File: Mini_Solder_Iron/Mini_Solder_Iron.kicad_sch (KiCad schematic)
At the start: 89 parts, among them CN1 YXT-BB10-24S-02, J1 USB_C_Receptacle_USB2.0, J2 Negative, J3 Positive, J4 Conn_01x04, J5 Conn_01x04, J6 Conn_01x04, J7 Com, J8 Conn_01x04, Q1 AO4407A, Q2 MMBT3904, SW1 SW_Push, SW2 SW_Push, U1 STM32F103C8T6, U2 LIS2DS12, U3 SGM8557-1AXN5G/TR, U4 TMP36GRTZ, U5 CH340E, U6 MP9942, U7 CH224K, U8 LP5907MFX-3.3, U9 LP5907MFX-1.8, Y1 Crystal_GND3_Small

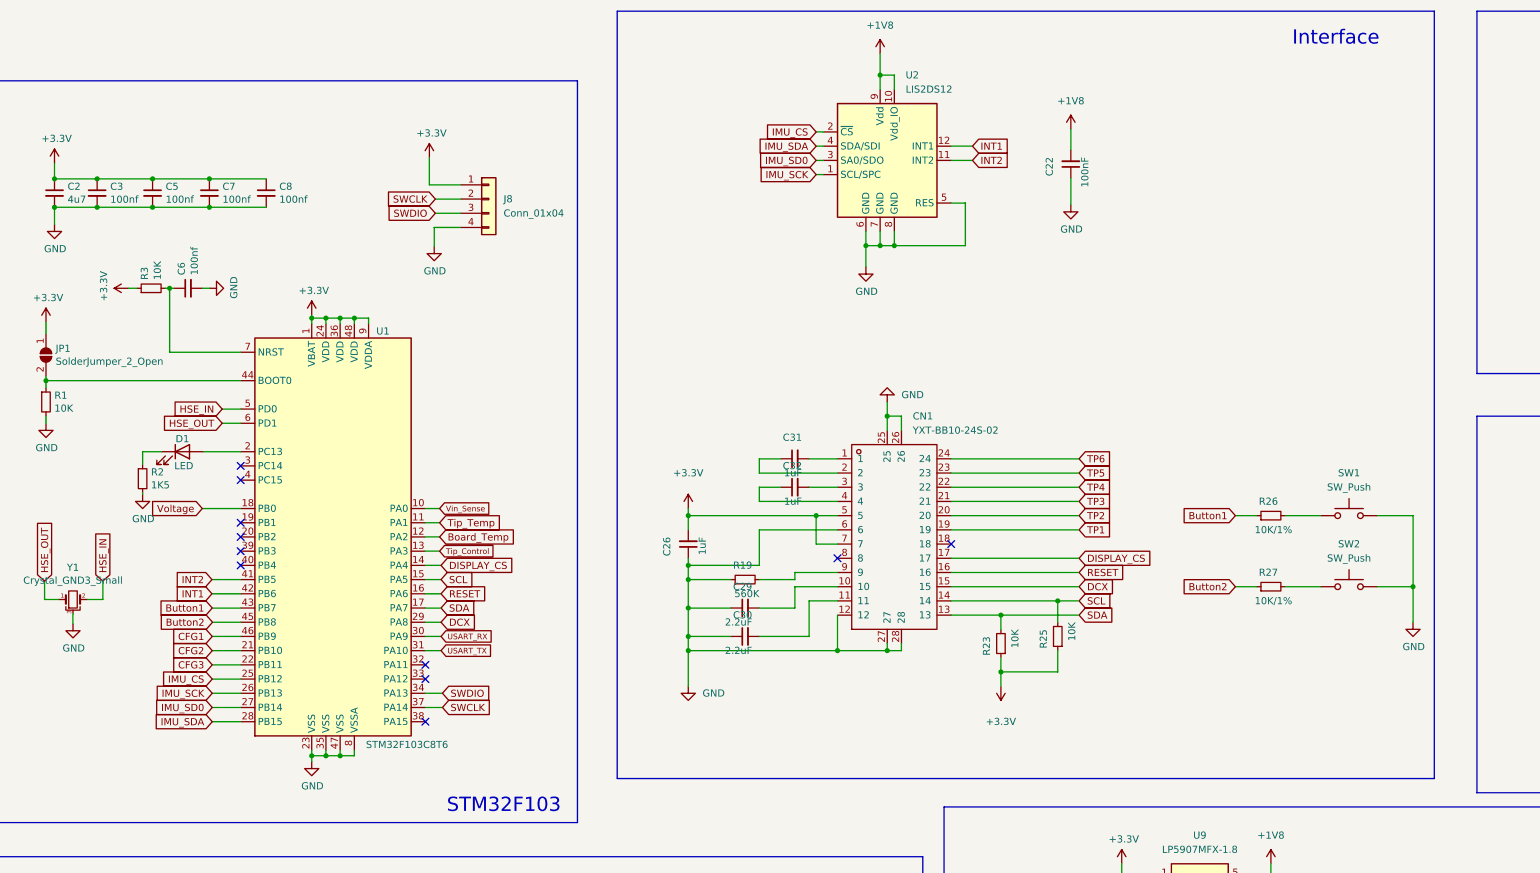
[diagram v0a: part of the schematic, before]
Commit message: PCB layout update
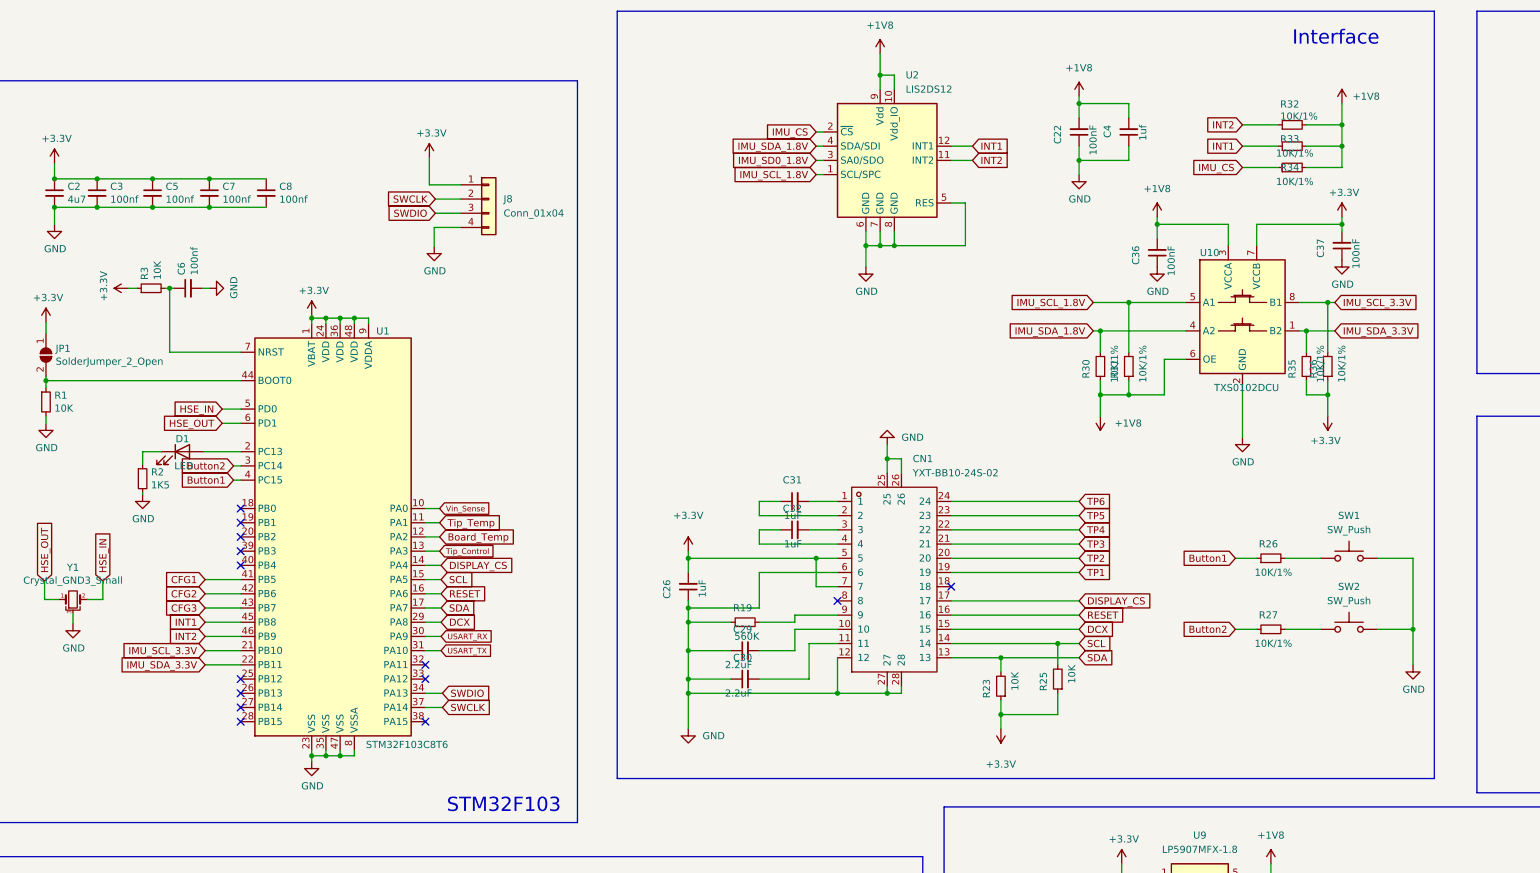
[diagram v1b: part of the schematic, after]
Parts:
- added C36, C37: 100nF, Capacitor_SMD:C_0402_1005Metric, symbol Device:C_Small
- added C4: 1uf, Capacitor_SMD:C_0402_1005Metric, symbol Device:C_Small
- added R30, R31, R32, R33, R34, R35, R36: 10K/1%, Resistor_SMD:R_0402_1005Metric, symbol Device:R_Small
- added U10: TXS0102DCU, Package_SO:VSSOP-8_2.3x2mm_P0.5mm, symbol Logic_LevelTranslator:TXS0102DCU
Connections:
- net +1V8: now also C36.2, C4.2, R30.1, R31.1, R32.2, R33.2, R34.2, U10.3 (VCCA), U10.6 (OE)
- net +3V3: now also C37.2, R35.1, R36.1, U10.7 (VCCB)
- net Button1: now also U1.4 (PC15); no longer U1.43 (PB7)
- net Button2: now also U1.3 (PC14); no longer U1.45 (PB8)
- net CFG1: now also U1.41 (PB5); no longer U1.46 (PB9)
- net CFG2: now also U1.42 (PB6); no longer U1.21 (PB10)
- net CFG3: now also U1.43 (PB7); no longer U1.22 (PB11)
- net GND: now also C36.1, C37.1, C4.1, U10.2 (GND)
- net IMU_CS: now also R34.1; no longer U1.25 (PB12)
- net INT1: now also U1.45 (PB8), R33.1; no longer U1.42 (PB6)
- net INT2: now also U1.46 (PB9), R32.1; no longer U1.41 (PB5)
- net Voltage: no longer U1.18 (PB0)
- net IMU_SCK: no longer names the net of U1.26 (PB13)
- net IMU_SCK: no longer U2.1 (SCL/SPC)
- net IMU_SD0: no longer names the net of U1.27 (PB14)
- net IMU_SD0: no longer U2.3 (SA0/SDO)
- net IMU_SDA: no longer names the net of U1.28 (PB15)
- net IMU_SDA: no longer U2.4 (SDA/SDI)
- new net IMU_SCL_1.8V: R31.2, U10.5 (A1), U2.1 (SCL/SPC)
- new net IMU_SCL_3.3V: R36.2, U1.21 (PB10), U10.8 (B1)
- new net IMU_SD0_1.8V: U2.3 (SA0/SDO)
- new net IMU_SDA_1.8V: R30.2, U10.4 (A2), U2.4 (SDA/SDI)
- new net IMU_SDA_3.3V: R35.2, U1.22 (PB11), U10.1 (B2)
- no-connect marks 17 -> 20
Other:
- moved on the sheet: C22, C26, C29, C30, C31, C32, CN1, R19, R23, R25, R26, R27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
